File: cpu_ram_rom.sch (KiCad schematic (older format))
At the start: 10 parts, among them SW2 Reset, U6 SRAM - IS62C5128BL-45TLI, U7 SST39SF040, U8 CPU -Z84C0020AEG, U9 DS1813R-5+T&R

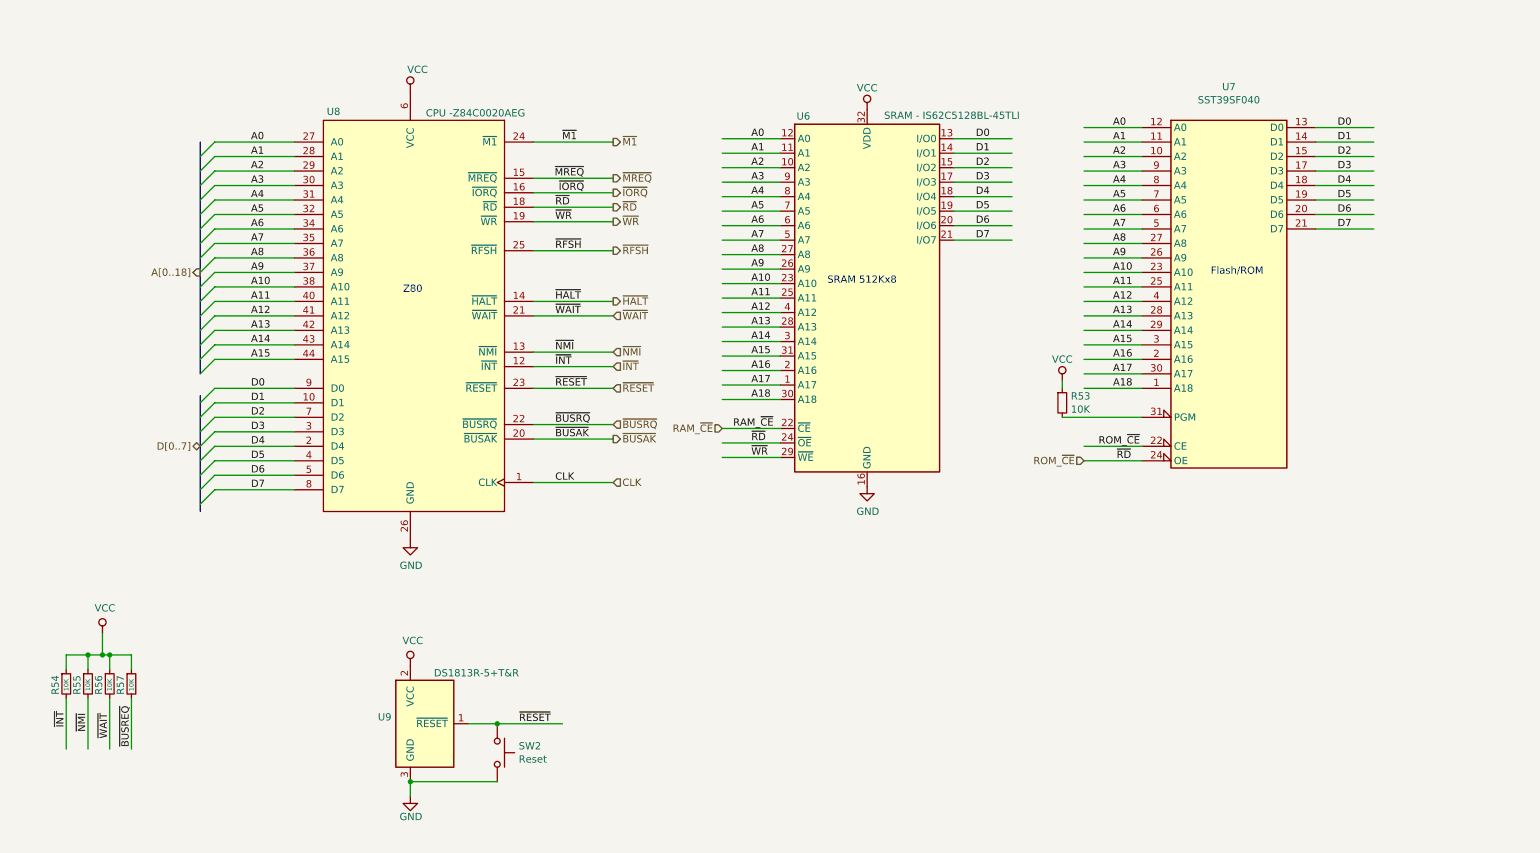
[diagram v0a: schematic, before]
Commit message: passed DRC
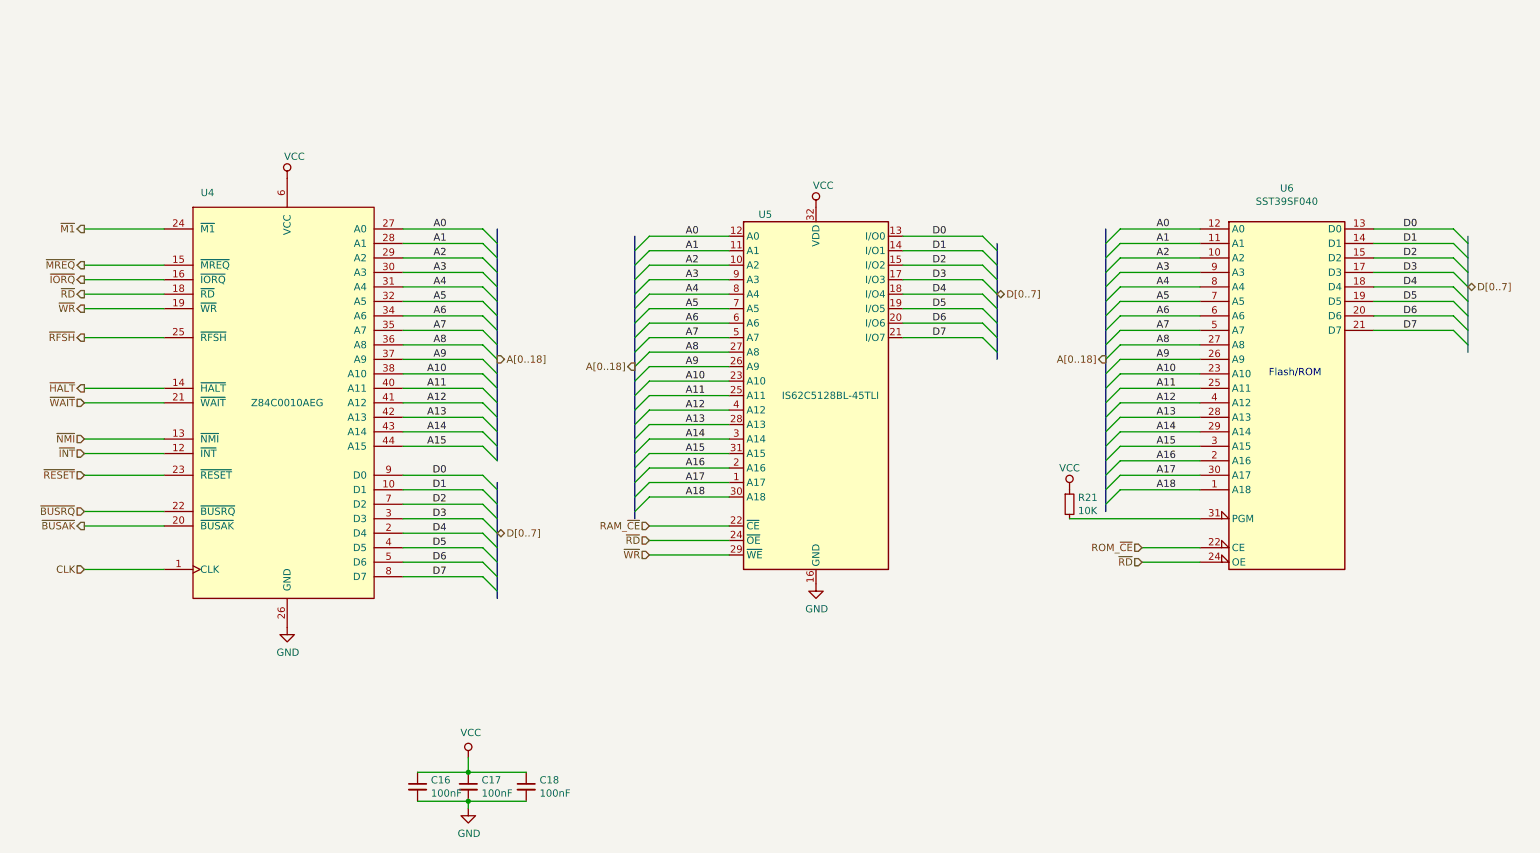
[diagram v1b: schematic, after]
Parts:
- removed R54, R55, R56, R57: 10K, Resistor_SMD:R_0603_1608Metric_Pad1.05x0.95mm_HandSolder, symbol Device:R_Small
- removed SW2: Reset, Button_Switch_SMD:SW_SPST_FSMSM, symbol Switch:SW_Push
- removed U6: SRAM - IS62C5128BL-45TLI, Package_SO:TSOP-II-32_21.0x10.2mm_P1.27mm, symbol THS-80:IS62C5128BL-45TLI
- removed U8: CPU -Z84C0020AEG, Package_QFP:LQFP-44_10x10mm_P0.8mm, symbol THS-80:Z84C0010AEG
- removed U9: DS1813R-5+T&R, Package_TO_SOT_SMD:SOT-23, symbol THS-80:DS1813R-5+T&R
- added C16, C17, C18: 100nF, Capacitor_SMD:C_0603_1608Metric_Pad1.05x0.95mm_HandSolder, symbol Device:C_Small
- added U4: Z84C0010AEG, Package_QFP:LQFP-44_10x10mm_P0.8mm, symbol THS-80:Z84C0010AEG
- added U5: IS62C5128BL-45TLI, Package_SO:TSOP-II-32_21.0x10.2mm_P1.27mm, symbol THS-80:IS62C5128BL-45TLI
- renumbered R53 to R21, U7 to U6
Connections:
- net labels removed: RAM_~CE, ~BUSREQ
- wire segments 116 -> 104
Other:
- note removed: "SRAM 512Kx8"
- note removed: "Z80"
- moved on the sheet: R21, U6

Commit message: finished routing, drc passed
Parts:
- added D13, D14: GRN, LED_SMD:LED_0603_1608Metric_Pad1.05x0.95mm_HandSolder, symbol Device:LED
- added R19, R20: 10K, Resistor_SMD:R_0603_1608Metric_Pad1.05x0.95mm_HandSolder, symbol Device:R_Small
- added R40, R41: 360R, Resistor_SMD:R_0603_1608Metric_Pad1.05x0.95mm_HandSolder, symbol Device:R_Small
- added U12: 74HCT3G04, Package_SO:TSSOP-8_3x3mm_P0.65mm, symbol 74xGxx:74HCT3G04
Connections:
- net labels added: RAM_~CE, ROM_~CE
- wire segments 104 -> 107
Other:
- moved on the sheet: C16, C17, C18, R21, U4, U5, U6
